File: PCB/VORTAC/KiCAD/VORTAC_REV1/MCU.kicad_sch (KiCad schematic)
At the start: 34 parts, among them IC1 TMC2209-LA, U2 STM32F103C8Tx, U6 SN65HVD232DR

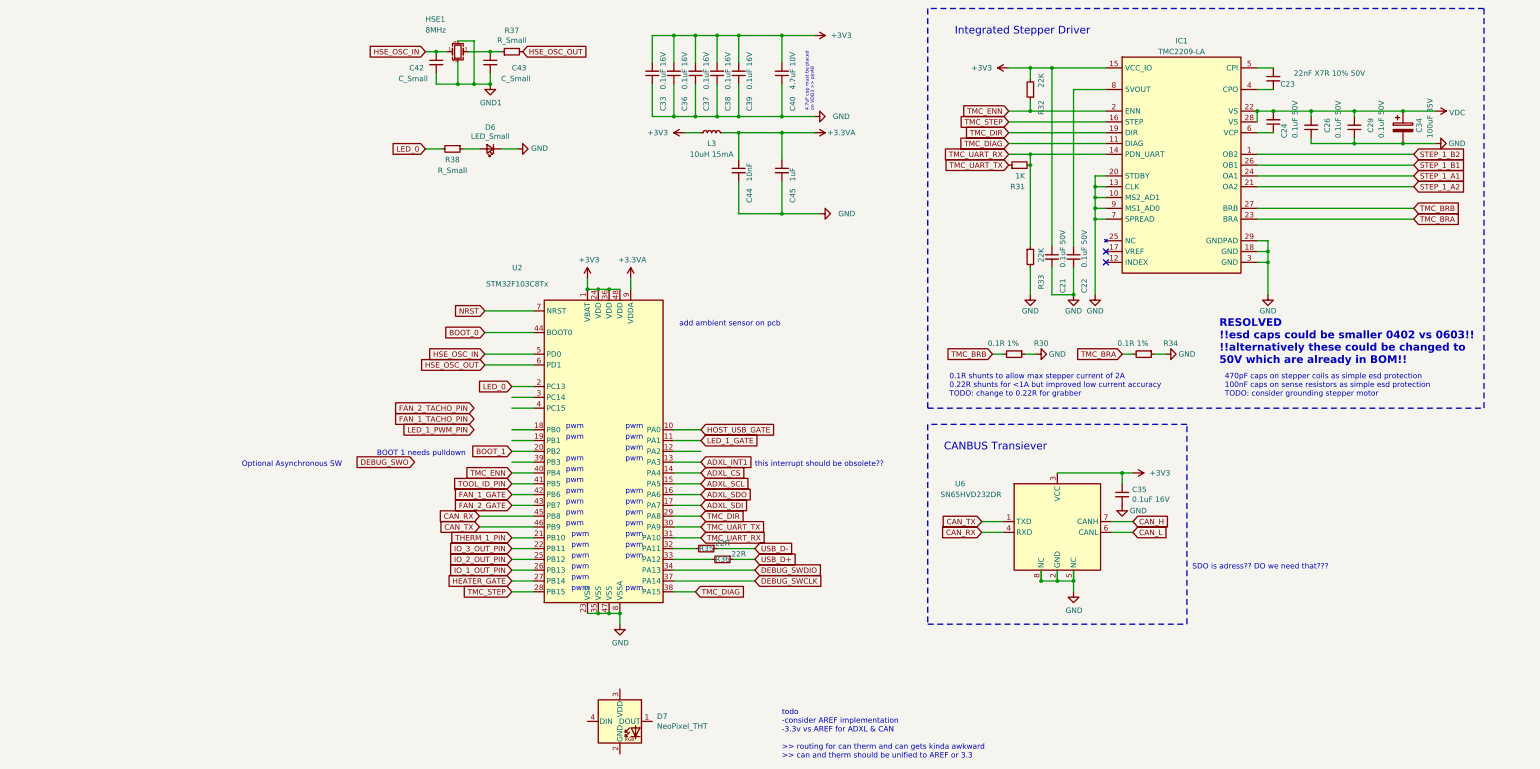
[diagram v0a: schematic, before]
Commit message: hallo
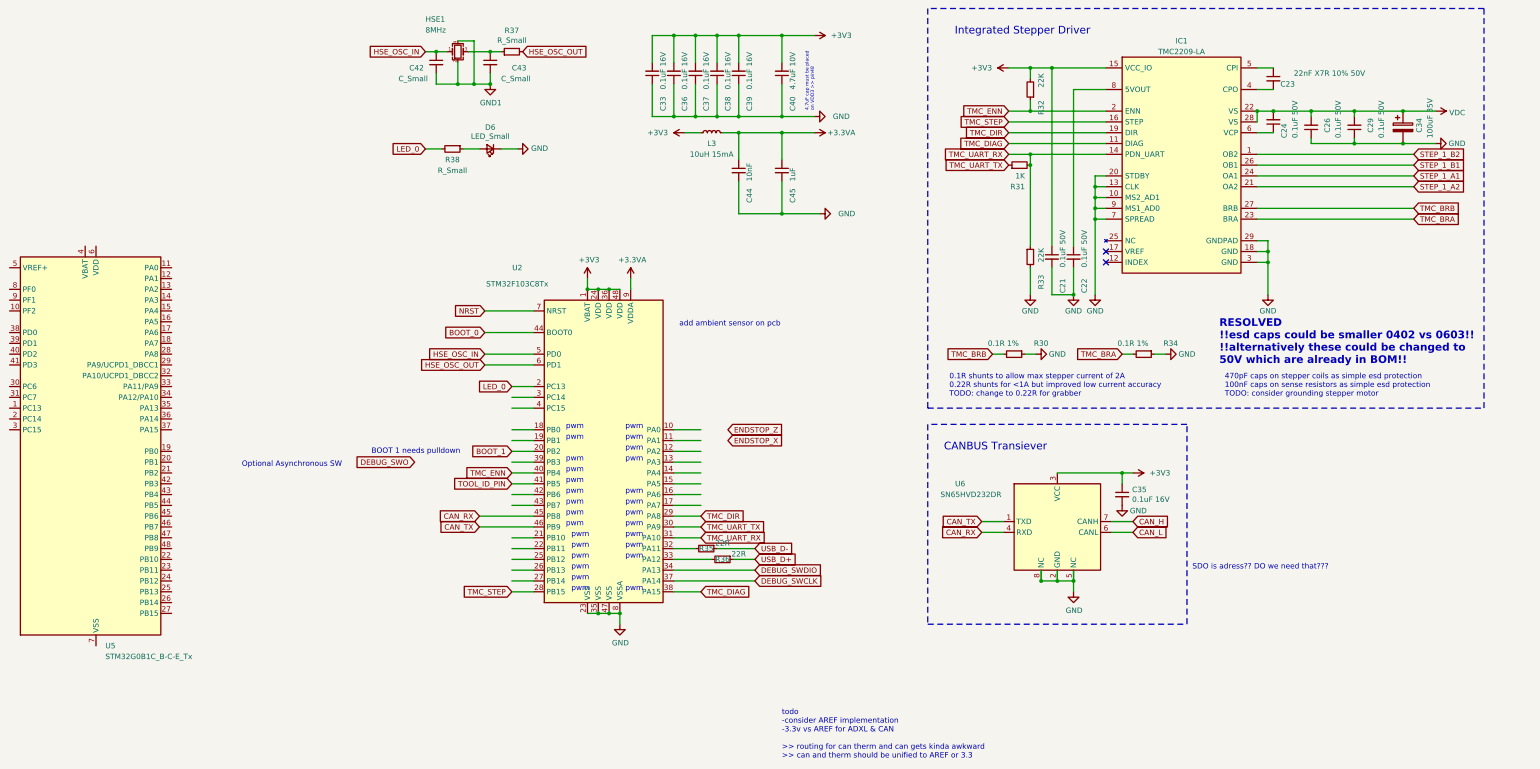
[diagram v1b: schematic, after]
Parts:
- removed D7: NeoPixel_THT, LED_SMD:LED_Cree-PLCC4_2x2mm_CW, symbol LED:NeoPixel_THT
- added U5: STM32G0B1C_B-C-E_Tx, Package_QFP:LQFP-48_7x7mm_P0.5mm, symbol MCU_ST_STM32G0:STM32G0B1C_B-C-E_Tx
- IC1: footprint ToolChanger:tmc_2209_ThermalPad -> ToolChanger:tmc_2209_package
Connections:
- net ADXL_CS: no longer names the net of U2.14 (PA4)
- net ADXL_INT1: no longer names the net of U2.13 (PA3)
- net ADXL_SCL: no longer names the net of U2.15 (PA5)
- net ADXL_SDI: no longer names the net of U2.17 (PA7)
- net ADXL_SDO: no longer names the net of U2.16 (PA6)
- net FAN_1_GATE: no longer names the net of U2.42 (PB6)
- net FAN_2_GATE: no longer names the net of U2.43 (PB7)
- net HEATER_GATE: no longer names the net of U2.27 (PB14)
- net HOST_USB_GATE: no longer names the net of U2.10 (PA0)
- net IO_1_OUT_PIN: no longer names the net of U2.26 (PB13)
- net IO_2_OUT_PIN: no longer names the net of U2.25 (PB12)
- net IO_3_OUT_PIN: no longer names the net of U2.22 (PB11)
- net LED_1_GATE: no longer names the net of U2.11 (PA1)
- net THERM_1_PIN: no longer names the net of U2.21 (PB10)
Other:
- note removed: "this interrupt should be obsolete??"

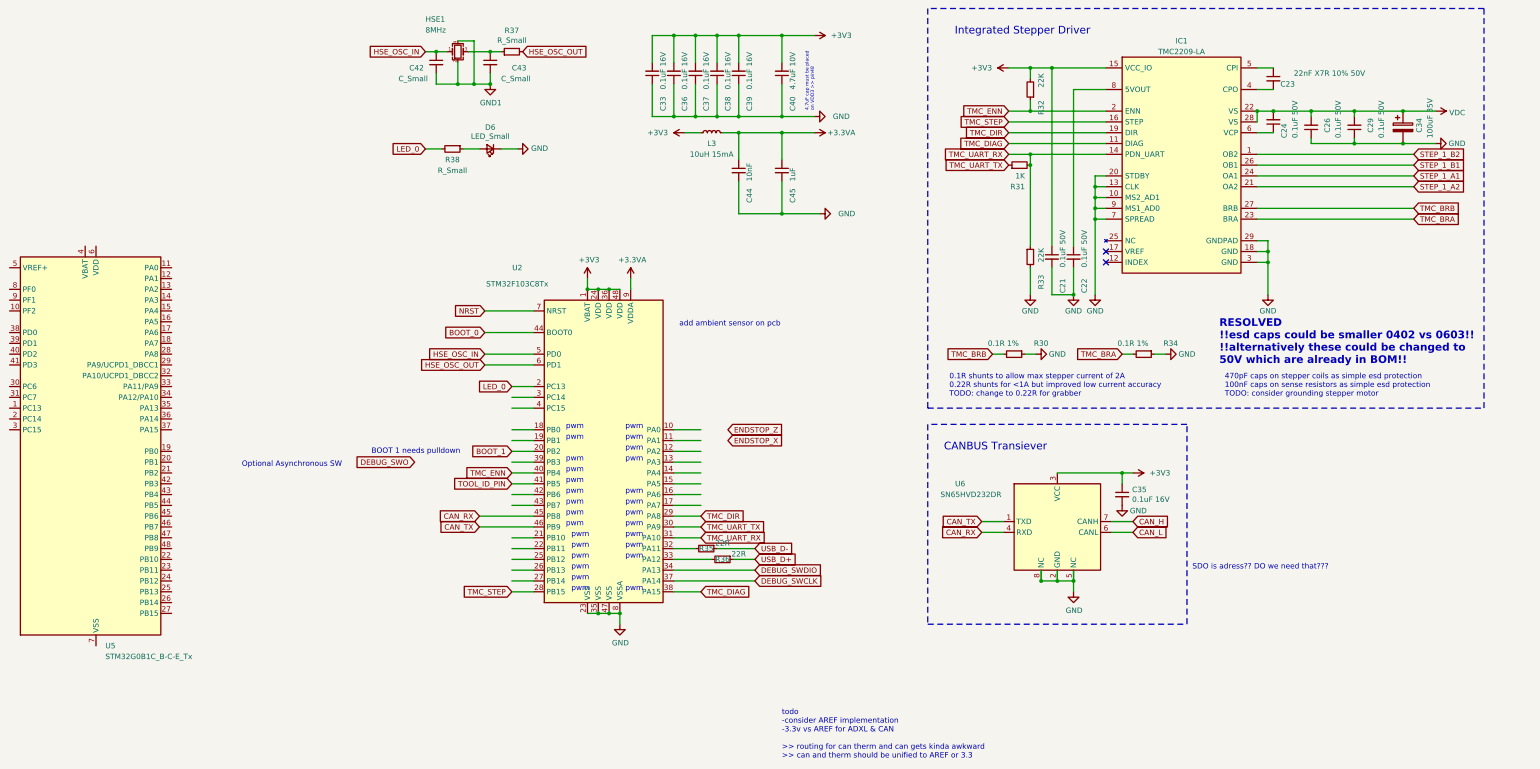
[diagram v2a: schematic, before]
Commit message: yipppieee
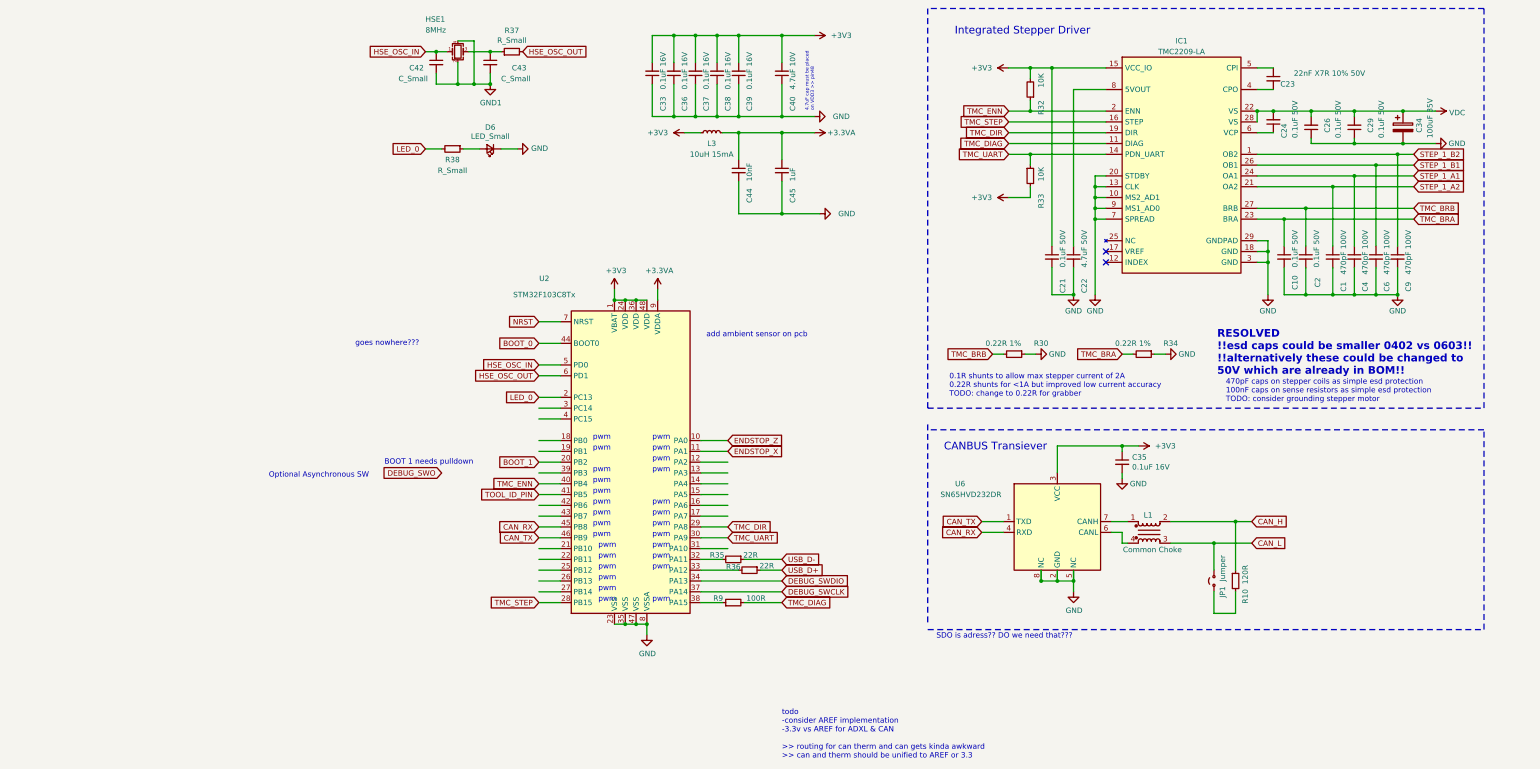
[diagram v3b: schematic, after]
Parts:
- removed R31: 1K, Resistor_SMD:R_0402_1005Metric, symbol Device:R_Small
- removed U5: STM32G0B1C_B-C-E_Tx, Package_QFP:LQFP-48_7x7mm_P0.5mm, symbol MCU_ST_STM32G0:STM32G0B1C_B-C-E_Tx
- added C1, C4, C6, C9: 470pF 100V, Capacitor_SMD:C_0603_1608Metric, symbol Device:C_Small
- added C10, C2: 0.1uF 50V, Capacitor_SMD:C_0603_1608Metric, symbol Device:C_Small
- added JP1: Jumper, Connector_PinHeader_1.27mm:PinHeader_2x01_P1.27mm_Vertical, symbol Jumper:Jumper_2_Small_Open
- added L1: Common Choke, Inductor_SMD:L_CommonModeChoke_Coilcraft_0805USB, symbol Filter:Choke_Wurth_WE-CNSW_744232090
- added R10: 120R, Resistor_SMD:R_0402_1005Metric, symbol Device:R_Small
- added R9: 100R, Resistor_SMD:R_0402_1005Metric, symbol Device:R_Small
- C22: value 0.1uF 50V -> 4.7uF 50V
- C34: footprint Capacitor_SMD:CP_Elec_8x6.9 -> Capacitor_SMD:CP_Elec_6.3x7.7; LCSC (none) -> C2983388
- R30, R34: value 0.1R 1% -> 0.22R 1%
- R32, R33: value 22K -> 10K
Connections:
- net TMC_UART_TX is gone; now on net TMC_UART: U2.30 (PA9)
- net +3V3: now also R33.2
- net CAN_H: now also L1.2, R10.1; no longer U6.7 (CANH)
- net CAN_L: now also JP1.2 (B), L1.3; no longer U6.6 (CANL)
- net ENDSTOP_X: now also U2.11 (PA1)
- net ENDSTOP_Z: now also U2.10 (PA0)
- net GND: now also C1.2, C10.2, C2.2, C4.2, C6.2, C9.2; no longer R33.2
- net STEP_1_A1: now also C4.1
- net STEP_1_A2: now also C1.1
- net STEP_1_B1: now also C6.1
- net STEP_1_B2: now also C9.1
- net TMC_BRA: now also C10.1
- net TMC_BRB: now also C2.1
- net TMC_DIAG: now also R9.2; no longer U2.38 (PA15)
- net TMC_UART_RX renamed TMC_UART
- net TMC_UART: no longer U2.31 (PA10)
- new net: R9.1, U2.38 (PA15)
- new net: L1.4, U6.6 (CANL)
- new net: L1.1, U6.7 (CANH)
- new net: JP1.1 (A), R10.2
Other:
- note added: "goes nowhere???"
- moved on the sheet: C35, R33, R35, R36, U2
